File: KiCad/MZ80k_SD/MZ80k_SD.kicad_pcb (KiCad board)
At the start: 2 copper layers, 100 x 100 mm, 18 parts, among them J1 MZ-80K BUS, J2 Micro_SD_Card_Kit, J3 INT VCC, J4 EXT 5V, U1 GAL22V10, U2 28C64, U3 8255, U4 Arduino_Pro_Mini_5V

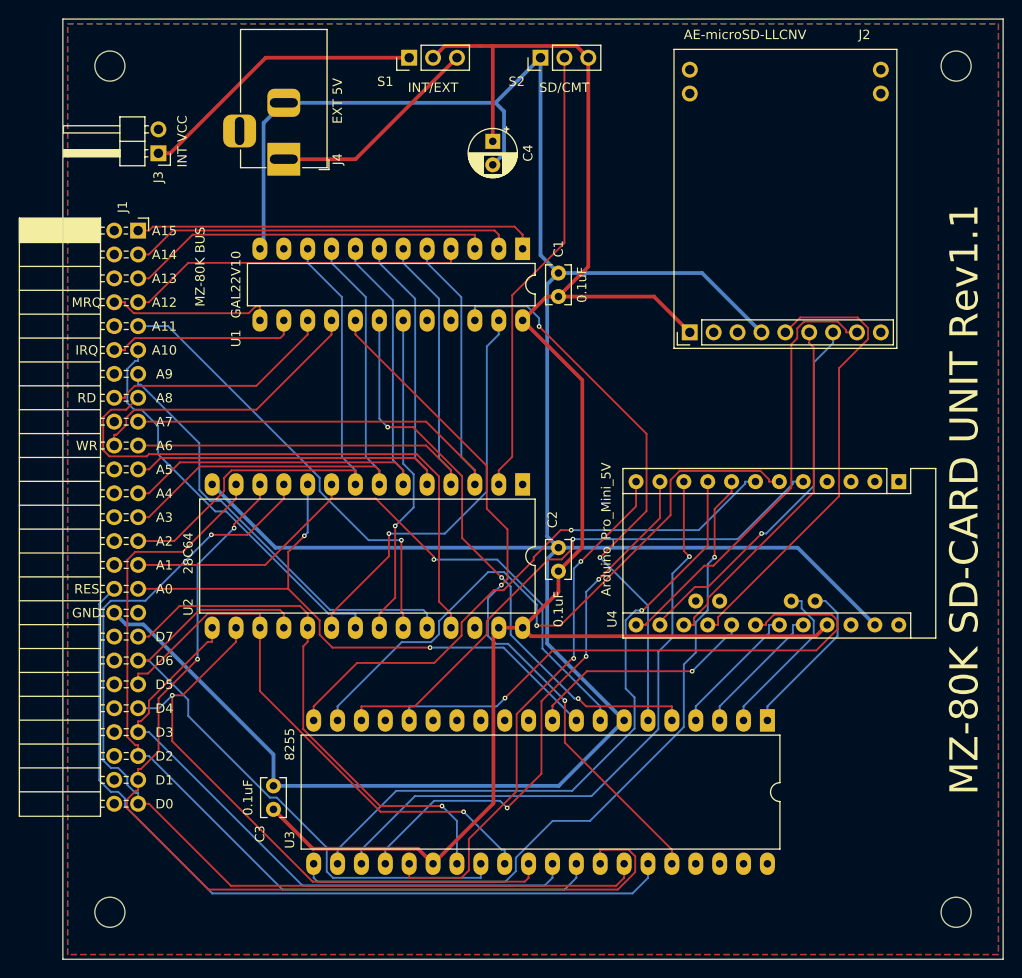
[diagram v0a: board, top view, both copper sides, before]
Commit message: Add files via upload
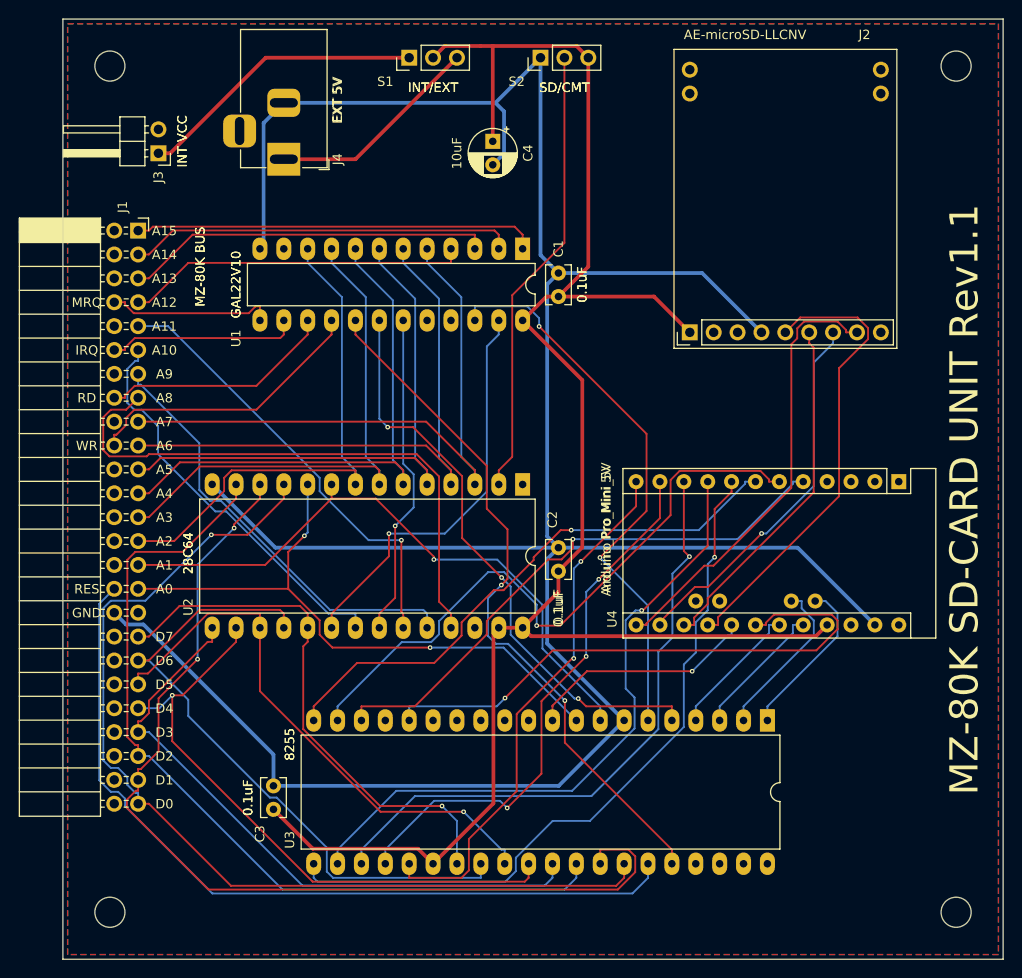
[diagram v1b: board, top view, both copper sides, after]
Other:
- board text added: "0.1uF"
- board text added: "10uF"
- board text added: "28C64"
- board text added: "8255"
- board text added: "Arduino Pro Mini 5V"
- board text added: "EXT 5V"
- board text added: "GAL22V10"
- board text added: "INT VCC"
- board text added: "INT/EXT"
- board text added: "MZ-80K BUS"
- board text added: "SD/CMT"
